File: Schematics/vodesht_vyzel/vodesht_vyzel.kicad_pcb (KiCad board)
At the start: 2 copper layers, 81.5 x 59 mm, 7 parts, among them U1 SSD1306, U2 NODEMCU32S, U3 NRF52840-DONGLE

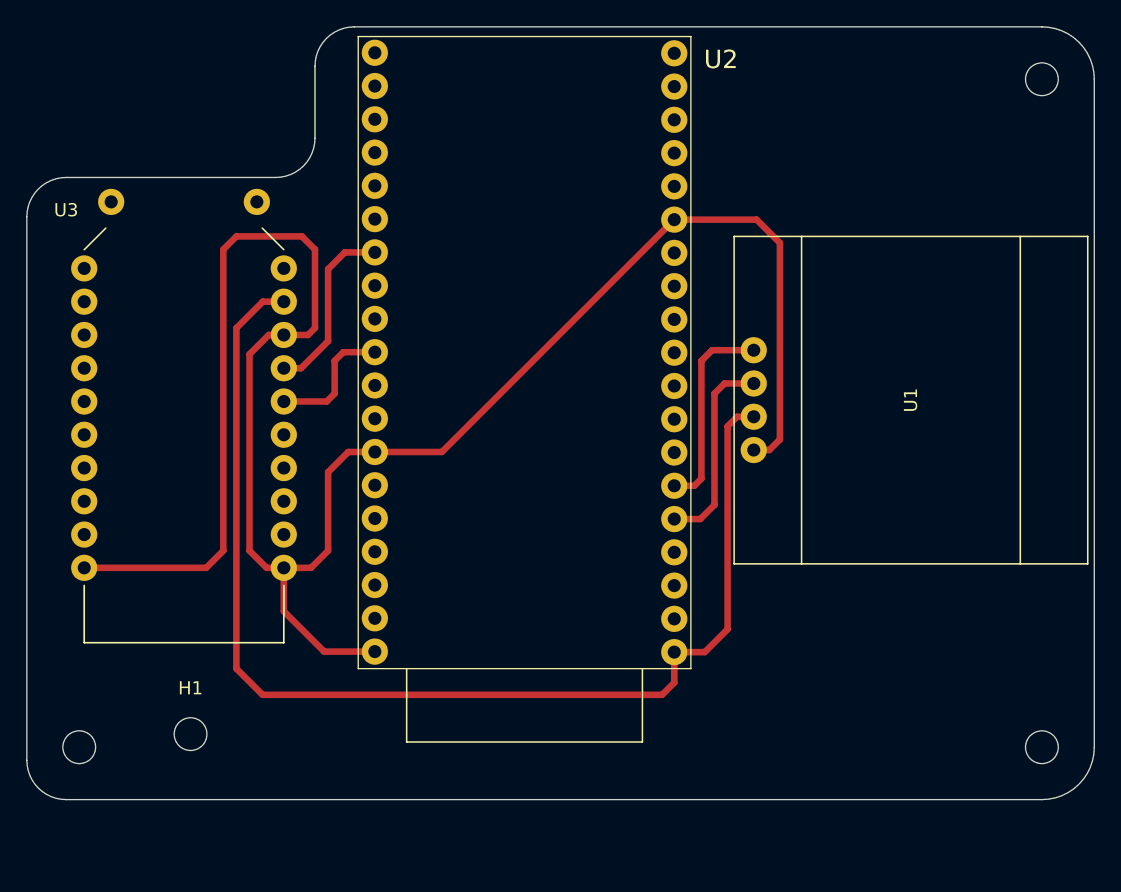
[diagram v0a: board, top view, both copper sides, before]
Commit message: Changes on the vodesht_vyzel pcb and schematics
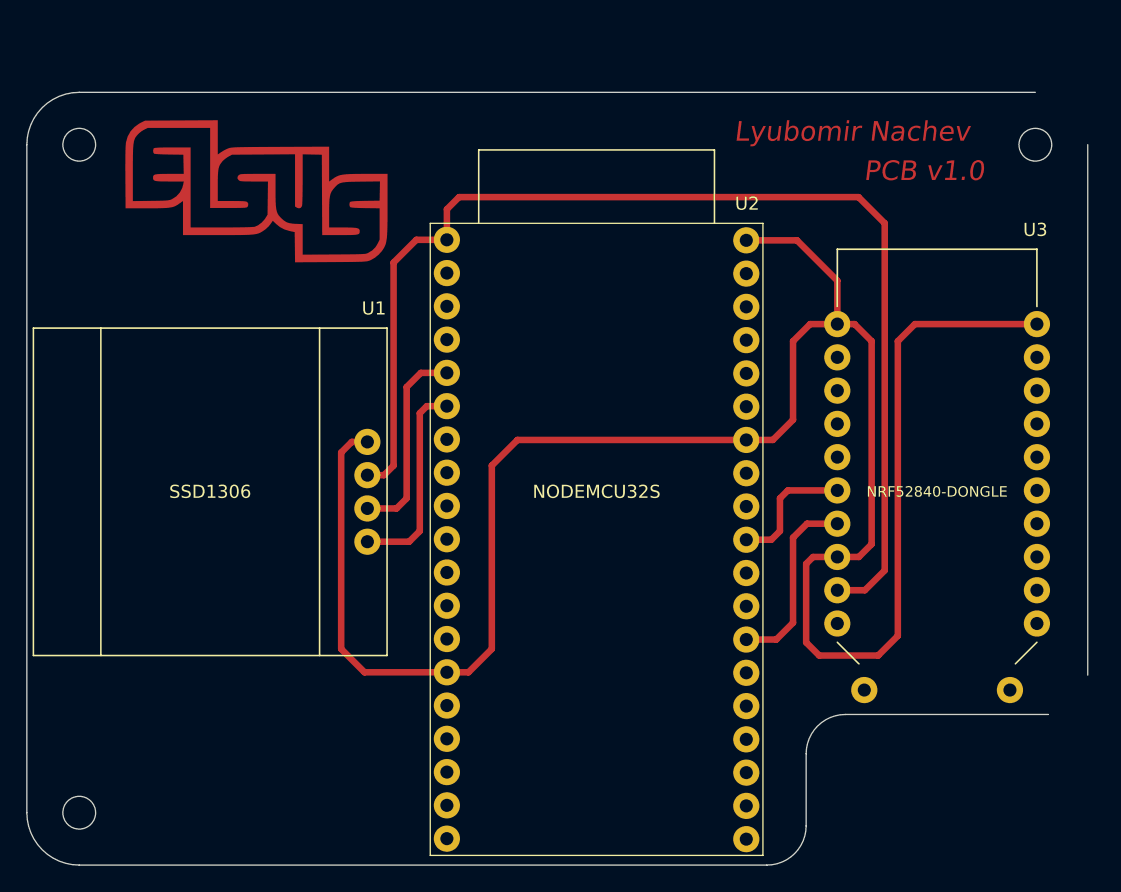
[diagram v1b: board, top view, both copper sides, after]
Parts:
- removed H4: MountingHole, MountingHole:MountingHole_2.5mm
- added G***: LOGO, LOGO, F.Cu at (132.5, 75.5)
- moved H2 92.4 mm to (119.0, 123.0), turned to 180 degrees
- moved H3 86.3 mm to (192.0, 72.0), turned to 180 degrees
- moved U3 59.7 mm to (184.5, 103.0), turned to -90 degrees
- moved U1 54.0 mm to (129.0, 98.5), turned to -90 degrees
- moved H1 45.8 mm to (119.0, 72.0)
- moved U2 19.8 mm to (158.5, 104.5), turned to 0 degrees
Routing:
- net GNDD: track 154.0 -> 162.2 mm
- net Net-(U2-Pad32): track 13.8 -> 14.4 mm
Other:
- board size 81.5 x 59 mm -> 81 x 59 mm
- board text added: "Lyubomir Nachev"
- board text added: "PCB v1.0"
